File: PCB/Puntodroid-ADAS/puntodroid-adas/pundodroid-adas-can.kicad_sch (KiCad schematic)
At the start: 12 parts, among them U6 SN65HVD230, U7 TJA1054

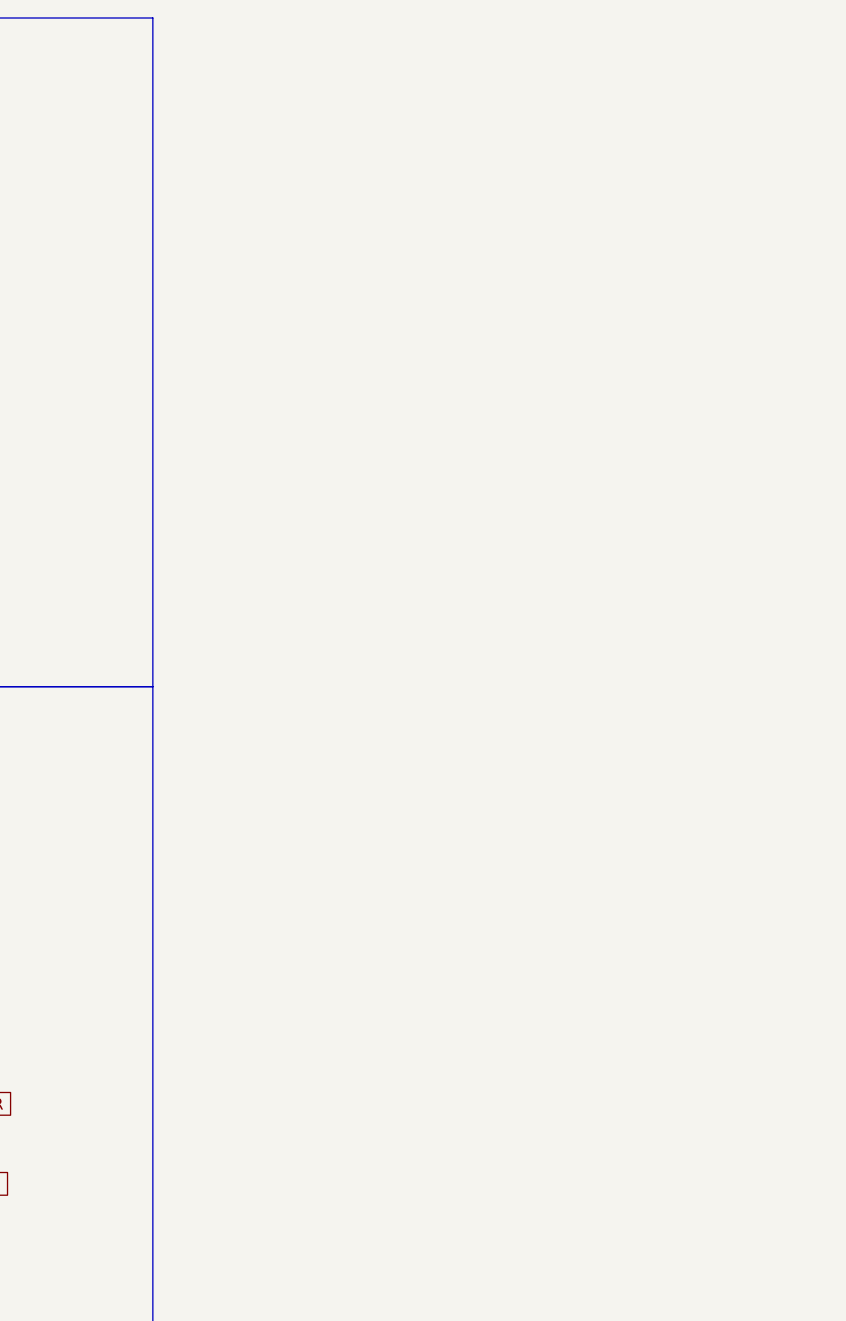
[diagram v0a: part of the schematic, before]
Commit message: update puntodroid schematic stm32
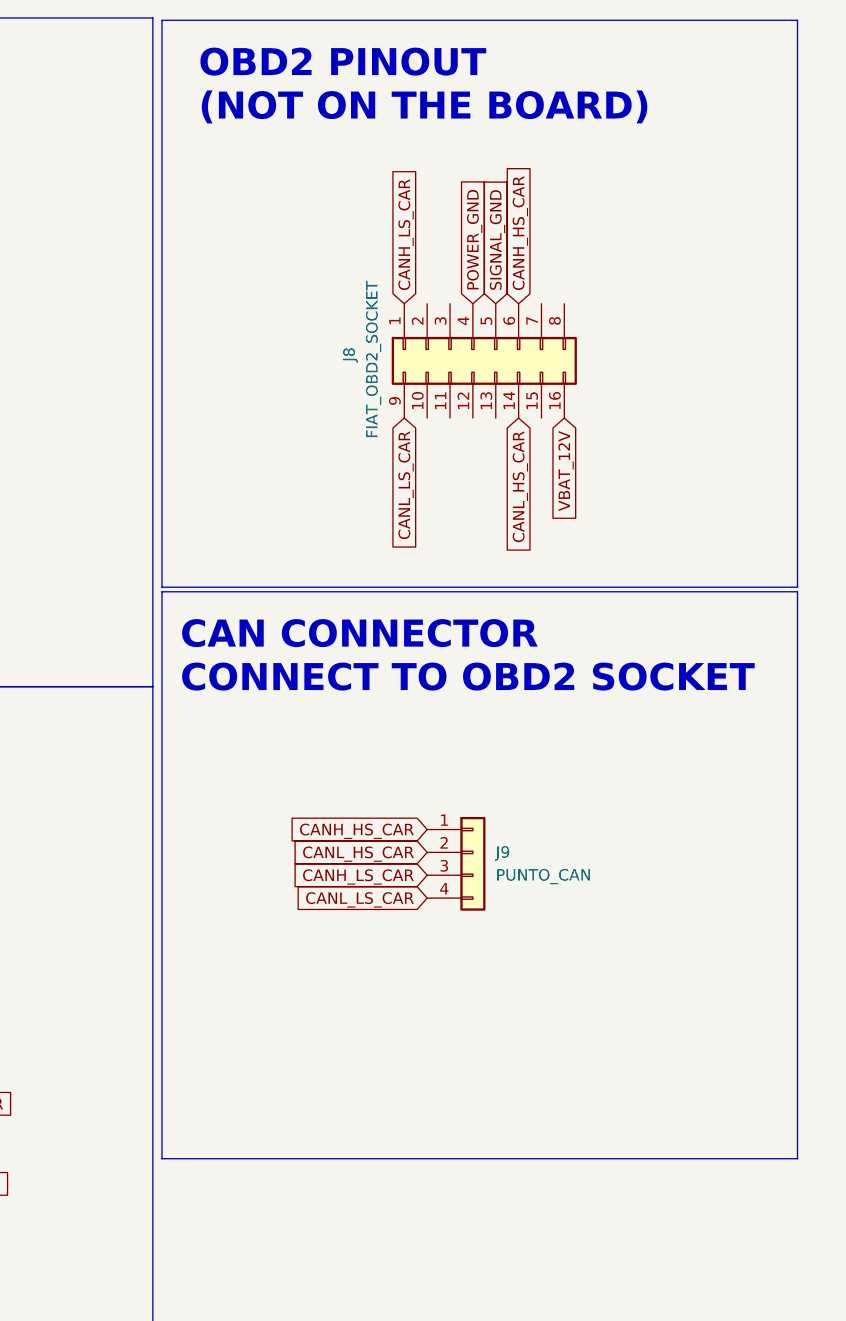
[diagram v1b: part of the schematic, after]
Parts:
- added J8: FIAT_OBD2_SOCKET, symbol Connector_Generic:Conn_02x08_Top_Bottom
- added J9: PUNTO_CAN, symbol Connector_Generic:Conn_01x04
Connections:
- net CANH_HS_CAR: now also J8.6 (Pin_6), J9.1 (Pin_1)
- net CANH_LS_CAR: now also J8.1 (Pin_1), J9.3 (Pin_3)
- net CANL_HS_CAR: now also J8.14 (Pin_14), J9.2 (Pin_2)
- net CANL_LS_CAR: now also J8.9 (Pin_9), J9.4 (Pin_4)
- new net POWER_GND: J8.4 (Pin_4)
- new net SIGNAL_GND: J8.5 (Pin_5)
- new net VBAT_12V: J8.16 (Pin_16)
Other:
- note added: "CAN CONNECTOR CONNECT TO OBD2 SOCKET"
- note added: "OBD2 PINOUT (NOT ON THE BOARD)"
